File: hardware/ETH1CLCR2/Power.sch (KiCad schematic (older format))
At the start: 43 parts, among them Q901 IRFR5410, U901 NMK0509SC, U902 NMK2405SAC, U903 MAX5902, U904 NCP1117-5.0_SOT223, U905 NMK2409SAC, U906 LT1175-5_SOT223, U907 NMK2409SC, U908 NCP1117-3.3_TO252, U909 NCP1117-5.0_TO252, U910 NCP1117-5.0_SOT223, U911 LT1175-5_SOT223

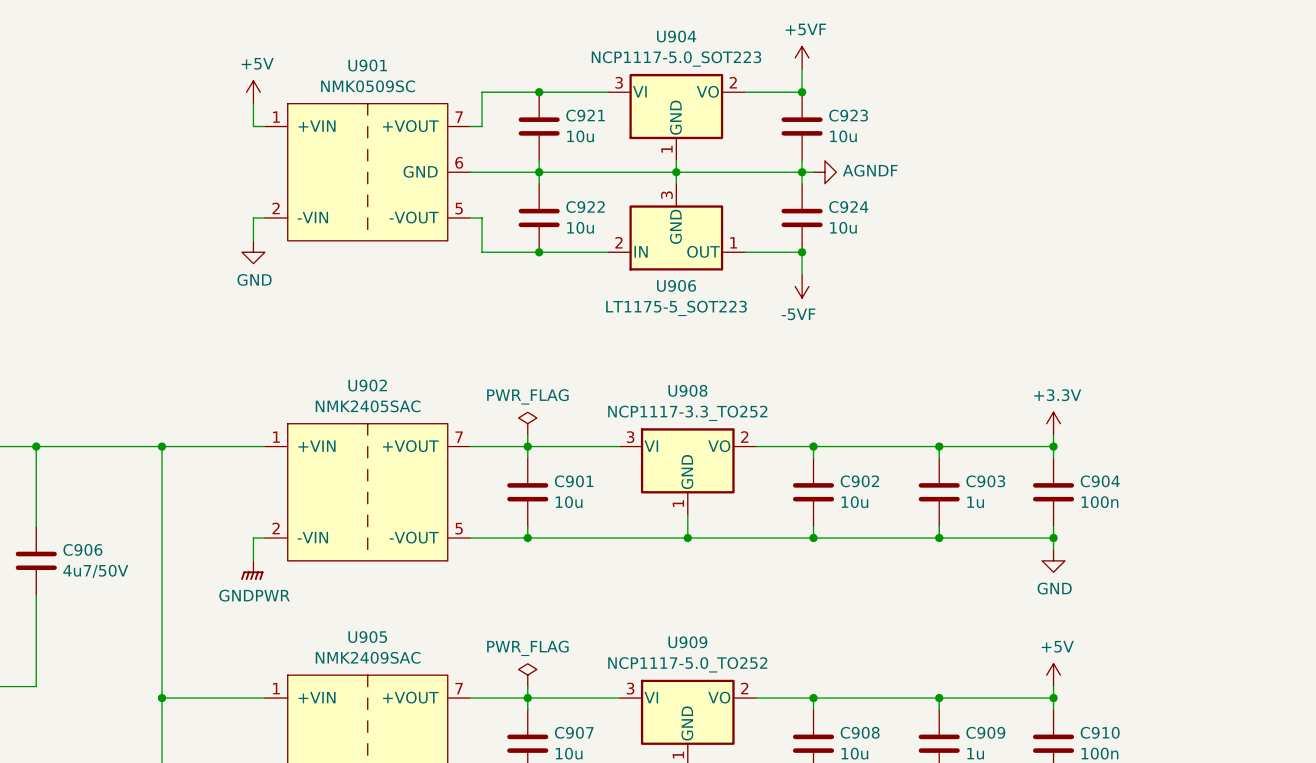
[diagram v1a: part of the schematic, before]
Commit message: Schematic
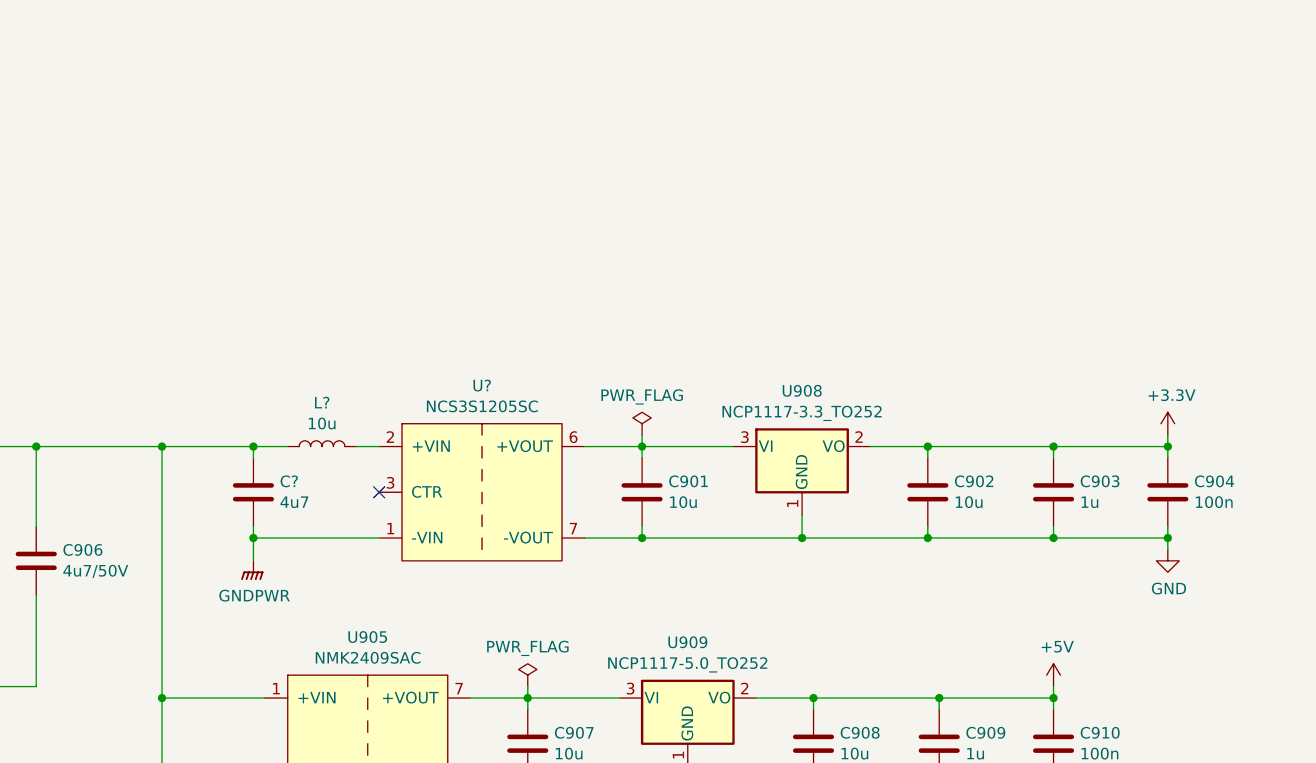
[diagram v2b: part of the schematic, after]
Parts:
- removed C921, C922, C923, C924: 10u, Capacitor_SMD:C_1206_3216Metric_Pad1.33x1.80mm_HandSolder, symbol Device:C
- removed U901: NMK0509SC, ETH1CLCR2:NMK_DUAL, symbol ETH1CLCR2:NMK_DUAL
- removed U902: NMK2405SAC, ETH1CLCR2:NMK_SINGLE, symbol ETH1CLCR2:NMK_SINGLE
- removed U904: NCP1117-5.0_SOT223, Package_TO_SOT_SMD:SOT-223-3_TabPin2, symbol Regulator_Linear:NCP1117-5.0_SOT223
- removed U906: LT1175-5_SOT223, Package_TO_SOT_SMD:SOT-223-3_TabPin2, symbol Regulator_Linear:LT1175-5_SOT223
- added C?: 4u7, symbol Device:C
- added L?: 10u, symbol Device:L
- added U?: NCS3S1205SC, symbol ETH1CLCR2:NCS3
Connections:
- net GND: now also U?.7 (-VOUT)
- net GNDPWR: now also C?.2, U?.1 (-VIN)
- net at C905.1, C906.1, D901.1 (K)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: now also C?.1, L?.1
- net at C901.1, U908.3 (VI): now also U?.6 (+VOUT)
- new net: L?.2, U?.2 (+VIN)
- no-connect marks 1 -> 2
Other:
- moved on the sheet: C901, C902, C903, C904, U908
